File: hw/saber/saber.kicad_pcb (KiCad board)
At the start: 2 copper layers, 115.6 x 61 mm, 81 parts, among them J1 Screw_Terminal_01x02, J2 Screw_Terminal_01x02, J3 Screw_Terminal_01x12, J4 NUCLEO144ZE-STLINK, Q1 STL120N4F6AG, Q2 SIS413DN-T1-GE3, Q3 SSM3K337R, Q4 STL76DN4LF7AG, Q5 SSM3K337R, Q6 SSM3K337R, Q7 SSM3K337R, SW1 SW, U1 STM32L031F4Px, U2 VNHD7008AY, U3 AZ1117IH-3.3TRG1, U4 MMA8452Q

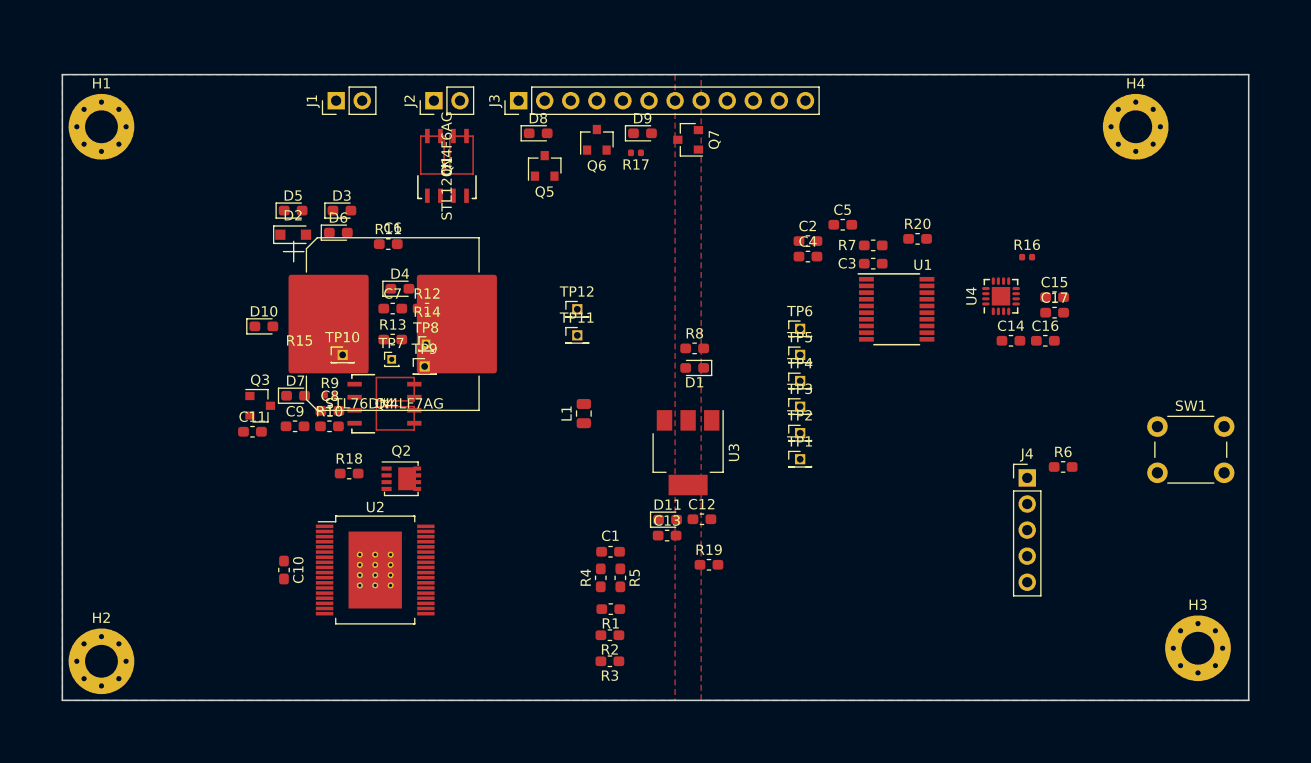
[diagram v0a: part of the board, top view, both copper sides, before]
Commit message: pre-datasheet-review placement
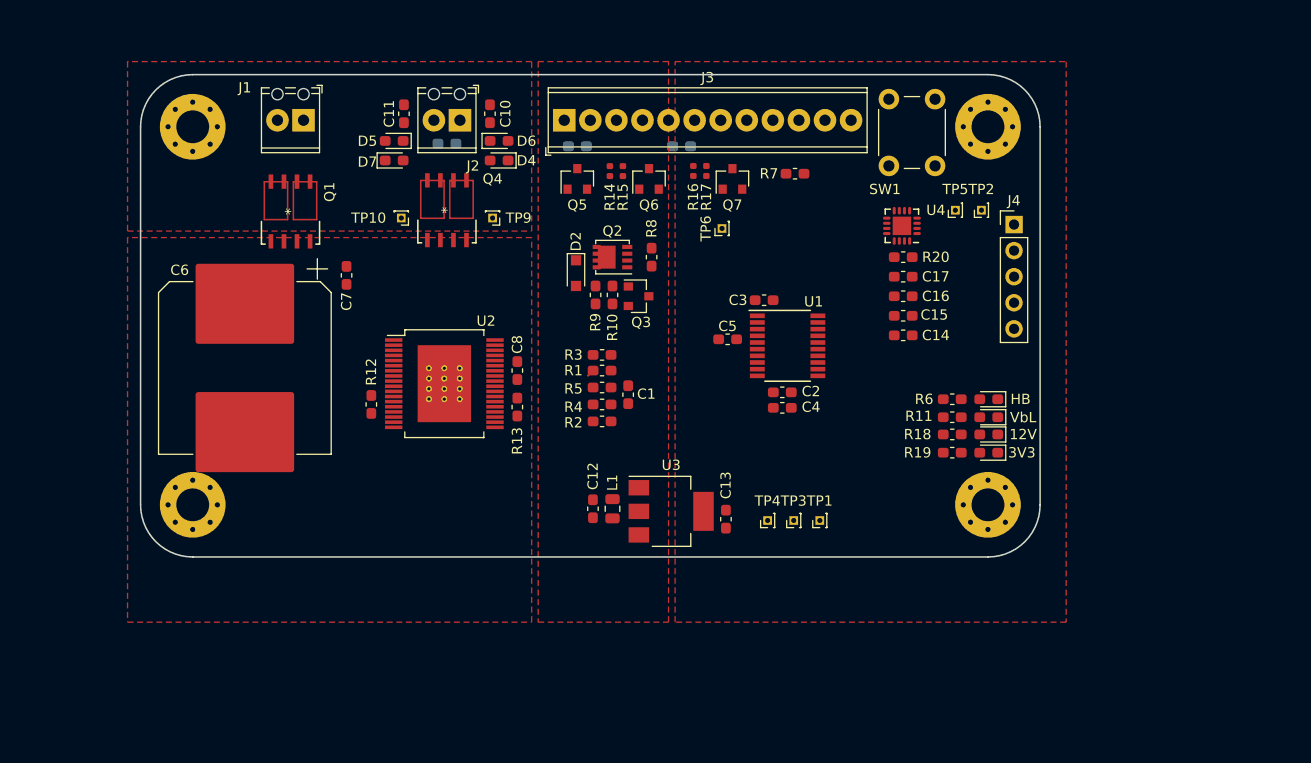
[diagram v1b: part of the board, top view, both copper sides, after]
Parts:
- removed TP11, TP12: TestPoint, Connector_PinHeader_1.27mm:PinHeader_1x01_P1.27mm_Vertical
- removed TP7, TP8: TestPoint, Connector_PinHeader_1.00mm:PinHeader_1x01_P1.00mm_Vertical
- C9, D8, D9: moved to B.Cu
- J1, J2: footprint Connector_PinHeader_2.54mm:PinHeader_1x02_P2.54mm_Vertical -> TerminalBlock_Phoenix:TerminalBlock_Phoenix_MPT-0,5-2-2.54_1x02_P2.54mm_Horizontal
- J3: footprint Connector_PinHeader_2.54mm:PinHeader_1x12_P2.54mm_Vertical -> TerminalBlock_Phoenix:TerminalBlock_Phoenix_MPT-0,5-12-2.54_1x12_P2.54mm_Horizontal
- Q1: value STL120N4F6AG -> (none)
- Q4: value STL76DN4LF7AG -> (none)
- R9: footprint Resistor_SMD:R_0402_1005Metric -> Resistor_SMD:R_0603_1608Metric_Pad1.05x0.95mm_HandSolder
- TP1, TP10, TP2, TP3, TP4, TP5, TP6, TP9: footprint Connector_PinHeader_1.27mm:PinHeader_1x01_P1.27mm_Vertical -> Connector_PinHeader_1.00mm:PinHeader_1x01_P1.00mm_Vertical
- moved 12V 71.4 mm to (185.5, 102.4), turned to 180 degrees
- moved VbL 66.1 mm to (185.5, 100.7), turned to 180 degrees
- moved R18 58.9 mm to (181.9, 102.4)
- moved R11 57.5 mm to (181.9, 100.7)
- moved C10 48.8 mm to (136.9, 71.1), turned to 90 degrees
- moved Q3 38.4 mm to (151.4, 88.9)
- moved SW1 36.5 mm to (175.8, 76.2), turned to 90 degrees
- moved R15 35.1 mm to (149.9, 76.7), turned to 90 degrees
- moved C11 34.3 mm to (128.5, 71.1), turned to 90 degrees
- moved R16 33.6 mm to (156.7, 76.7), turned to 270 degrees
- moved 3V3 32.0 mm to (185.5, 104.1), turned to 180 degrees
- moved C9 31.3 mm to (132.7, 74.0), turned to 180 degrees
- moved R10 30.4 mm to (148.8, 88.8), turned to 270 degrees
- moved R3 29.9 mm to (147.8, 94.6)
- moved Q2 29.8 mm to (148.8, 85.1), turned to 180 degrees
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- renumbered D10 to 12V, D11 to 3V3, H1 to ?, H2 to ?, H3 to ?, H4 to ?, D1 to HB, D3 to VbL
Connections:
- net Net-(C6-Pad1) renamed /hbridge/VCC
- Q4 pad 5: /MOT+ -> /MOT-
- Q4 pad 6: /MOT+ -> /MOT-
- Q4 pad 7: /MOT- -> /MOT+
- Q4 pad 8: /MOT- -> /MOT+
- TP10 pad 1: Net-(Q4-Pad4) -> Net-(Q4-Pad2)
- TP9 pad 1: Net-(Q4-Pad2) -> Net-(Q4-Pad4)
- U2 pad 13: Net-(Q4-Pad4) -> Net-(Q4-Pad2)
- U2 pad 24: Net-(Q4-Pad2) -> Net-(Q4-Pad4)
- U4 pad 10: (no net) -> GND
- U4 pad 11: Net-(U4-Pad11) -> /acc/SCL
- U4 pad 2: Net-(C17-Pad2) -> Net-(R20-Pad1)
- U4 pad 4: /acc/SCL -> Net-(U4-Pad4)
- U4 pad 6: /acc/SDA -> Net-(U4-Pad6)
- U4 pad 7: Net-(R20-Pad1) -> Net-(C17-Pad2)
- U4 pad 9: Net-(U4-Pad9) -> /acc/SDA
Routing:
- net /hbridge/PWM_MTR: track 0.00 -> 0.71 mm
- net /hbridge/imtr: track 0.00 -> 0.68 mm
- added copper zone on F.Cu, net /BATT+
- added copper zone on F.Cu, net /hbridge/VCC
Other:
- board size 115.6 x 61 mm -> 87.6 x 47 mm
